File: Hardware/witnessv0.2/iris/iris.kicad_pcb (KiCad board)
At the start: 4 copper layers, 30 x 50 mm, 112 parts, among them J1 Conn_01x02, J2 Conn_01x02, J3 USB_B_Micro, J4 Conn_01x02, J5 Conn_01x04, J6 Conn_01x04, J7 Conn_01x04, J8 Conn_01x04, J9 Conn_01x04, Q1 SQA403EJ, Q2 SQA403EJ, U1 ESP32-S3FN8, U10 RA-01SH-P, U2 TPS63070, U3 INA2180A3IDSG, U4 LSM6DSV320XTR, U5 ICM-45686, U6 TPS63070, U7 MS5607-02BA, U8 W25N01KVZEIR, U9 USBLC6-2SC6, Y1 F322540MUBCE2O

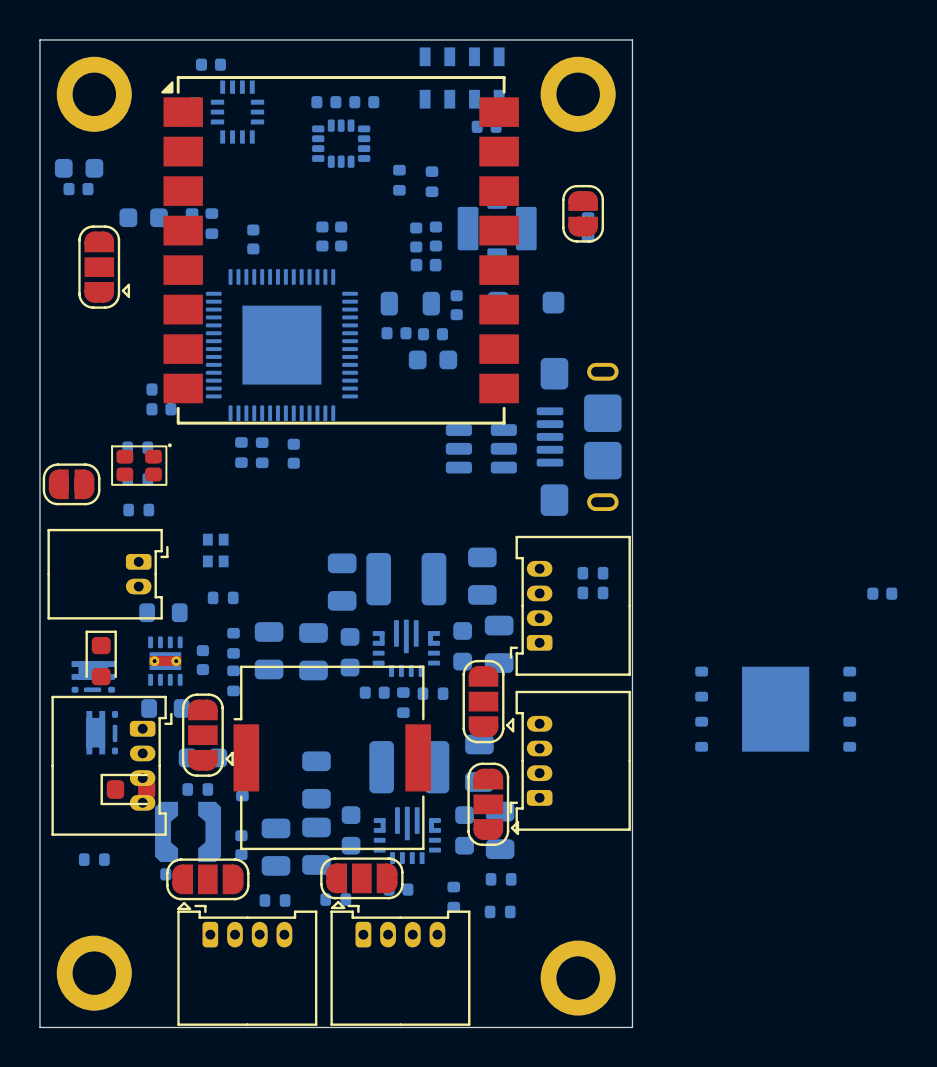
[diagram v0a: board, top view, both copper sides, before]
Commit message: iris rework
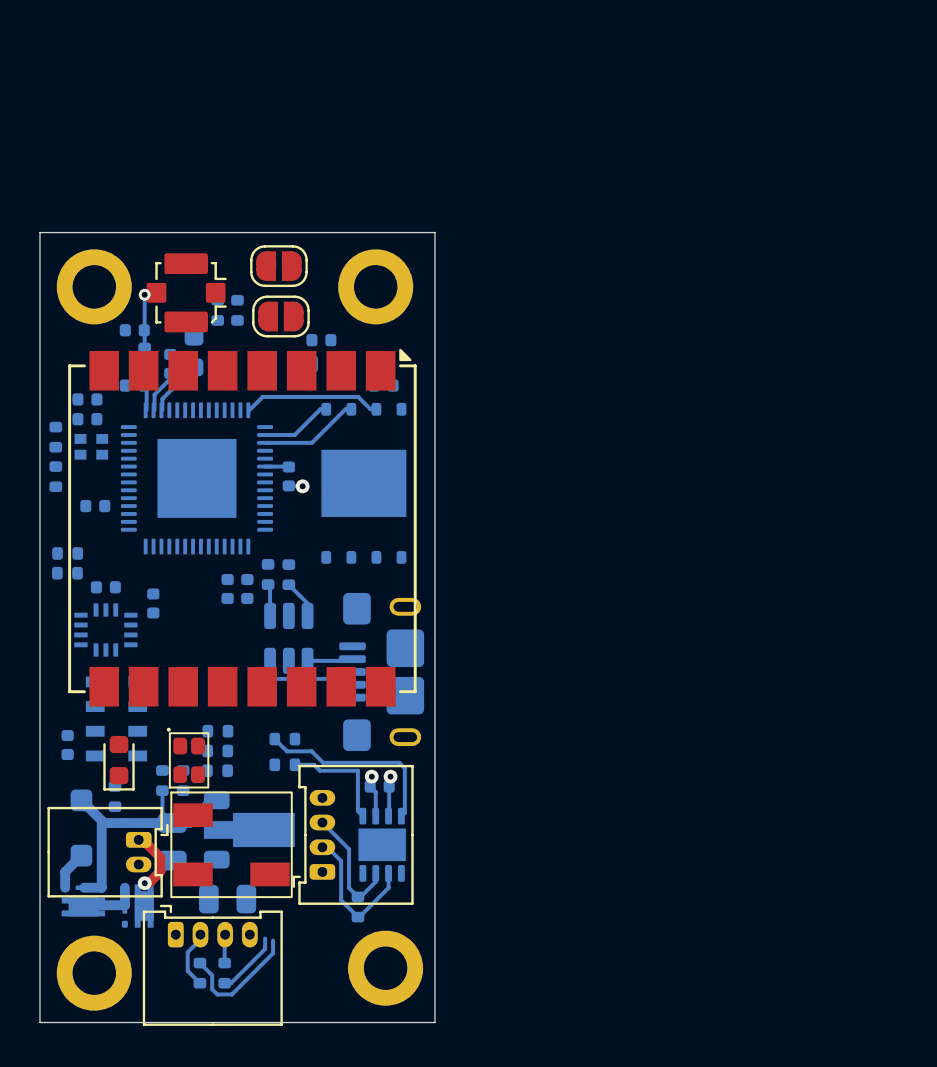
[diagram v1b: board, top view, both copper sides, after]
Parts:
- removed C12, C13, C14, C23, C24, C25: 22u, Capacitor_SMD:C_0805_2012Metric
- removed C15, C16, C21, C29, C34, C39, C40, C7: 100n, Capacitor_SMD:C_0402_1005Metric
- removed C17: 470n, Capacitor_SMD:C_0603_1608Metric
- removed C18, C19: 10u, Capacitor_SMD:C_0805_2012Metric
- removed C20, C22, C43, C8, C9: 10u, Capacitor_SMD:C_0603_1608Metric
- removed D3: LED, LED_SMD:LED_0603_1608Metric
- removed J7, J8, J9: Conn_01x04, Witness:Molex_MicroLock-2200980471-01x04-Horizontal
- removed JP1, JP2, JP3, JP4, JP5, JP6: SolderJumper_3_Open, Jumper:SolderJumper-3_P1.3mm_Open_RoundedPad1.0x1.5mm
- removed L1, L3: 1u, Inductor_SMD:L_1210_3225Metric
- removed L2: 2.2u, Inductor_SMD:L_Coilcraft_LPS3010
- removed L4: 10n, Inductor_SMD:L_0805_2012Metric
- removed R1, R9: 100k, Resistor_SMD:R_0402_1005Metric
- removed R10, R12, R6: 10k, Resistor_SMD:R_0402_1005Metric
- removed R11: 35k, Resistor_SMD:R_0402_1005Metric
- removed R2: 470k, Resistor_SMD:R_0402_1005Metric
- removed R3: 150k, Resistor_SMD:R_0402_1005Metric
- removed R5: 4.7, Resistor_SMD:R_0402_1005Metric
- removed R7: 680k, Resistor_SMD:R_0402_1005Metric
- removed R8: 130k, Resistor_SMD:R_0402_1005Metric
- removed U3: INA2180A3IDSG, Package_SON:Texas_DSG0008A_WSON-8-1EP_2x2mm_P0.5mm_EP0.9x1.6mm_ThermalVias
- removed U6: TPS63070, Witness:RNM0015A
- added R32: 1k, Resistor_SMD:R_0402_1005Metric, B.Cu at (110.2, 126.5)
- added R35: 0, Resistor_SMD:R_0402_1005Metric, B.Cu at (111.1, 136.2)
- added R36: 0, Resistor_SMD:R_0402_1005Metric, B.Cu at (112.3, 136.2)
- added R39: 120, Resistor_SMD:R_0402_1005Metric, B.Cu at (119.1, 132.9)
- AE1: moved to F.Cu
- BZ1: footprint Buzzer_Beeper:Buzzer_Murata_PKMCS0909E -> Witness:OWMB-505020S-40-12D
- R33, R34: value 2.5m -> 0; footprint Resistor_SMD:R_0603_1608Metric -> Resistor_SMD:R_0402_1005Metric
- U2: value TPS63070 -> ME6118A33PG; footprint Witness:RNM0015A -> Package_TO_SOT_SMD:SOT-89-3
- U5: value ICM-45686 -> TCAN1044A-Q1; footprint Package_LGA:LGA-14_3x2.5mm_P0.5mm_LayoutBorder3x4y -> Package_SON:VSON-8-1EP_3x3mm_P0.65mm_EP1.65x2.4mm
- moved C38 37.8 mm to (104.4, 124.7), turned to 90 degrees
- moved U7 36.9 mm to (106.9, 123.4), turned to 0 degrees
- moved U5 35.6 mm to (120.3, 129.8), turned to -90 degrees
- moved D4 34.8 mm to (105.1, 128.9), turned to -90 degrees
- moved C36 27.4 mm to (108.7, 117.5), turned to 90 degrees
- moved C35 27.4 mm to (120.4, 106.5)
- moved U4 27.1 mm to (106.3, 118.9), turned to 0 degrees
- moved C37 24.5 mm to (106.3, 116.7), turned to 0 degrees
- moved R25 24.2 mm to (103.8, 111.1)
- moved U8 23.8 mm to (119.4, 111.5), turned to 90 degrees
- moved R28 23.2 mm to (112.0, 102.7), turned to 90 degrees
- moved R29 23.0 mm to (113.0, 102.7), turned to -90 degrees
- moved C28 23.0 mm to (120.2, 126.8), turned to 180 degrees
- moved R24 21.7 mm to (103.8, 109.1), turned to -90 degrees
- moved R27 18.8 mm to (104.4, 116.0), turned to 0 degrees
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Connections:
- net Net-(J3-D+) renamed /IO/USB_UNSAFE_D+
- net Net-(J3-D-) renamed /IO/USB_UNSAFE_D-
- C10 pad 1: /Power/BATT_POSTSW -> +BATT
- C11 pad 1: /Power/BATT_POSTSW -> +3V3
- C28 pad 1: Net-(C28-Pad1) -> +3V3
- D4 pad 1: Net-(D4-K) -> +BATT
- J2 pad 1: +BATT -> /IO/BATT_RAW
- J5 pad 1: Net-(J5-Pin_1) -> +3V3
- J6 pad 1: Net-(J6-Pin_1) -> /IO/GPIO
- J6 pad 2: /IO/GPIO1 -> /IO/CAN_L
- J6 pad 3: /IO/GPIO2 -> /IO/CAN_H
- Q1 pad 1: Net-(D4-K) -> /IO/BATT_RAW
- Q1 pad 4: /Power/ISENSE+ -> Net-(Q1-S)
- Q2 pad 1: +BATT -> Net-(Q1-S)
- Q2 pad 4: Net-(D4-K) -> +BATT
- R21 pad 1: GND -> /MCU/VSENSE
- R21 pad 2: Net-(D3-K) -> +BATT
- R30 pad 1: /MCU/USB_D- -> /IO/USB_D-
- R31 pad 1: /MCU/USB_D+ -> /IO/USB_D+
- R33 pad 1: /Power/ISENSE+ -> /MCU/CANTX
- R33 pad 2: /Power/BATT_POSTSW -> /IO/CANTX
- R34 pad 1: /Power/5VSENSE+ -> /MCU/CANRX
- R34 pad 2: +5V -> /IO/CANRX
- U1 pad 10: unconnected-(U1-GPIO5-Pad10) -> /MCU/RXD_MCU
- U1 pad 11: unconnected-(U1-GPIO6-Pad11) -> /MCU/RAD_RST
- U1 pad 12: unconnected-(U1-GPIO7-Pad12) -> /MCU/LSM_INT1
- U1 pad 13: unconnected-(U1-GPIO8-Pad13) -> /MCU/LSM_INT2
- U1 pad 14: unconnected-(U1-GPIO9-Pad14) -> /MCU/SPI2_IO3
- U1 pad 15: unconnected-(U1-GPIO10-Pad15) -> /MCU/FLASH_CS
- U1 pad 16: unconnected-(U1-GPIO11-Pad16) -> /MCU/SPI2_IO0
- U1 pad 17: unconnected-(U1-GPIO12-Pad17) -> /MCU/SPI2_CLK
- U1 pad 18: unconnected-(U1-GPIO13-Pad18) -> /MCU/SPI2_IO1
- U1 pad 19: unconnected-(U1-GPIO14-Pad19) -> /MCU/SPI2_IO2
- U1 pad 2: Net-(C28-Pad1) -> +3V3
- U1 pad 21: unconnected-(U1-XTAL_32K_P-Pad21) -> /MCU/SPI3_SCLK
- U1 pad 22: unconnected-(U1-XTAL_32K_N-Pad22) -> /MCU/RAD_CS
- U1 pad 23: unconnected-(U1-GPIO17-Pad23) -> /MCU/SPI3_COPI
- U1 pad 24: unconnected-(U1-GPIO18-Pad24) -> /MCU/SPI3_CIPO
- U1 pad 27: unconnected-(U1-GPIO21-Pad27) -> /MCU/MS56_CS
- U1 pad 3: Net-(C28-Pad1) -> +3V3
- U1 pad 36: unconnected-(U1-SPICLK_N-Pad36) -> /MCU/BUZZER
- U1 pad 37: unconnected-(U1-SPICLK_P-Pad37) -> /MCU/LED_B
- U1 pad 38: unconnected-(U1-GPIO33-Pad38) -> /MCU/I2C_SDA
- U1 pad 39: unconnected-(U1-GPIO34-Pad39) -> /MCU/I2C_SCL
- U1 pad 40: unconnected-(U1-GPIO35-Pad40) -> /MCU/LSM_CS
- U1 pad 41: unconnected-(U1-GPIO36-Pad41) -> /MCU/CANTX
- U1 pad 42: unconnected-(U1-GPIO37-Pad42) -> /MCU/CANRX
- U1 pad 43: unconnected-(U1-GPIO38-Pad43) -> /IO/GPIO
- U1 pad 44: unconnected-(U1-MTCK-Pad44) -> /MCU/RAD_BUSY
- U1 pad 45: unconnected-(U1-MTDO-Pad45) -> /MCU/RAD_RF_EN
- U1 pad 47: unconnected-(U1-MTDI-Pad47) -> /MCU/LED_R
- U1 pad 48: unconnected-(U1-MTMS-Pad48) -> /MCU/LED_G
- U1 pad 6: unconnected-(U1-GPIO1-Pad6) -> /MCU/VSENSE
- U1 pad 7: unconnected-(U1-GPIO2-Pad7) -> /MCU/RAD_DIO1
- U1 pad 9: unconnected-(U1-GPIO4-Pad9) -> /MCU/TXD_MCU
- U10 pad 10: /Radio/RAD_BUSY -> /MCU/RAD_BUSY
- U10 pad 11: /Radio/RAD_RF_EN -> /MCU/RAD_RF_EN
- U10 pad 12: /Radio/SPI1_SCLK -> /MCU/SPI3_SCLK
- U10 pad 13: /Radio/SPI1_CIPO -> /MCU/SPI3_CIPO
- U10 pad 14: /Radio/SPI1_COPI -> /MCU/SPI3_COPI
- U10 pad 15: /Radio/RAD_CS -> /MCU/RAD_CS
- U10 pad 4: /Radio/RAD_RST -> /MCU/RAD_RST
- U10 pad 5: Net-(JP6-C) -> +3V3
- U10 pad 6: /Radio/RAD_DIO1 -> /MCU/RAD_DIO1
- U2 pad 1: Net-(U2-PS/SYNC) -> GND
- U2 pad 2: Net-(U2-PG) -> +3V3
- U2 pad 3: Net-(U2-VAUX) -> +BATT
- U4 pad 1: /Sensors/SPI1_CIPO -> /MCU/SPI3_CIPO
- U4 pad 12: /Sensors/LSM_CS -> /MCU/LSM_CS
- U4 pad 13: /Sensors/I2C_SCL -> /MCU/I2C_SCL
- U4 pad 14: /Sensors/I2C_SDA -> /MCU/I2C_SDA
- U4 pad 2: /Sensors/SPI1_SCLK -> /MCU/SPI3_SCLK
- U4 pad 3: /Sensors/SPI1_COPI -> /MCU/SPI3_COPI
- U4 pad 4: /Sensors/LSM_INT1 -> /MCU/LSM_INT1
- U4 pad 9: /Sensors/LSM_INT2 -> /MCU/LSM_INT2
- U5 pad 1: /Sensors/SPI1_CIPO -> /IO/CANRX
- U5 pad 2: /Sensors/I2C_SDA -> GND
- U5 pad 3: /Sensors/I2C_SCL -> +3V3
- U5 pad 4: /Sensors/ICM_INT1 -> /IO/CANTX
- U5 pad 5: +3V3 -> unconnected-(U5-NC-Pad5)
- U5 pad 6: GND -> /IO/CAN_L
- U5 pad 7: unconnected-(U5-RESV-Pad7) -> /IO/CAN_H
- U5 pad 8: +3V3 -> unconnected-(U5-STB-Pad8)
- U5 pad 9: /Sensors/ICM_INT2 -> (no net)
- U7 pad 4: /Sensors/MS56_CS -> /MCU/MS56_CS
- U7 pad 5: /Sensors/MS56_CS -> /MCU/MS56_CS
- U7 pad 6: /Sensors/SPI1_CIPO -> /MCU/SPI3_CIPO
- U7 pad 7: /Sensors/SPI1_COPI -> /MCU/SPI3_COPI
- U7 pad 8: /Sensors/SPI1_SCLK -> /MCU/SPI3_SCLK
- U8 pad 2: /MCU/SPI3_IO2 -> /MCU/SPI2_IO1
- U8 pad 3: /MCU/SPI3_IO3 -> /MCU/SPI2_IO2
- U8 pad 5: /MCU/SPI2_IO1 -> /MCU/SPI2_IO0
- U8 pad 7: /MCU/SPI3_IO3 -> /MCU/SPI2_IO3
- U8 pad 9: (no net) -> GND
- U9 pad 3: /IO/USB_D+ -> /IO/USB_D-
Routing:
- net +BATT: track 0.00 -> 13.9 mm
- net /IO/CANTX: track 0.00 -> 9.69 mm
- net +3V3: track 0.00 -> 8.29 mm, vias 0 -> 1
- net /IO/CAN_L: track 0.00 -> 7.32 mm
- net /MCU/SPI2_IO3: track 0.00 -> 6.97 mm
- net /MCU/TXD_MCU: track 0.00 -> 6.28 mm
- net /IO/CAN_H: track 0.00 -> 6.15 mm
- net /IO/CANRX: track 0.00 -> 5.72 mm
- net /IO/USB_UNSAFE_D+: track 0.00 -> 5.09 mm
- net /MCU/SPI2_CLK: track 0.00 -> 5.02 mm
- net /MCU/SPI2_IO0: track 0.00 -> 3.58 mm
- net /MCU/RXD_MCU: track 0.00 -> 3.30 mm
- net /IO/BATT_RAW: track 0.00 -> 3.22 mm, vias 0 -> 1
- net Net-(Q1-S): track 0.00 -> 3.02 mm
- net /IO/TXD_MCU: track 0.00 -> 2.98 mm
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- added copper zone on In1.Cu, net +3V3
- added copper zone on In2.Cu, net GND
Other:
- board size 30 x 50 mm -> 20 x 40 mm

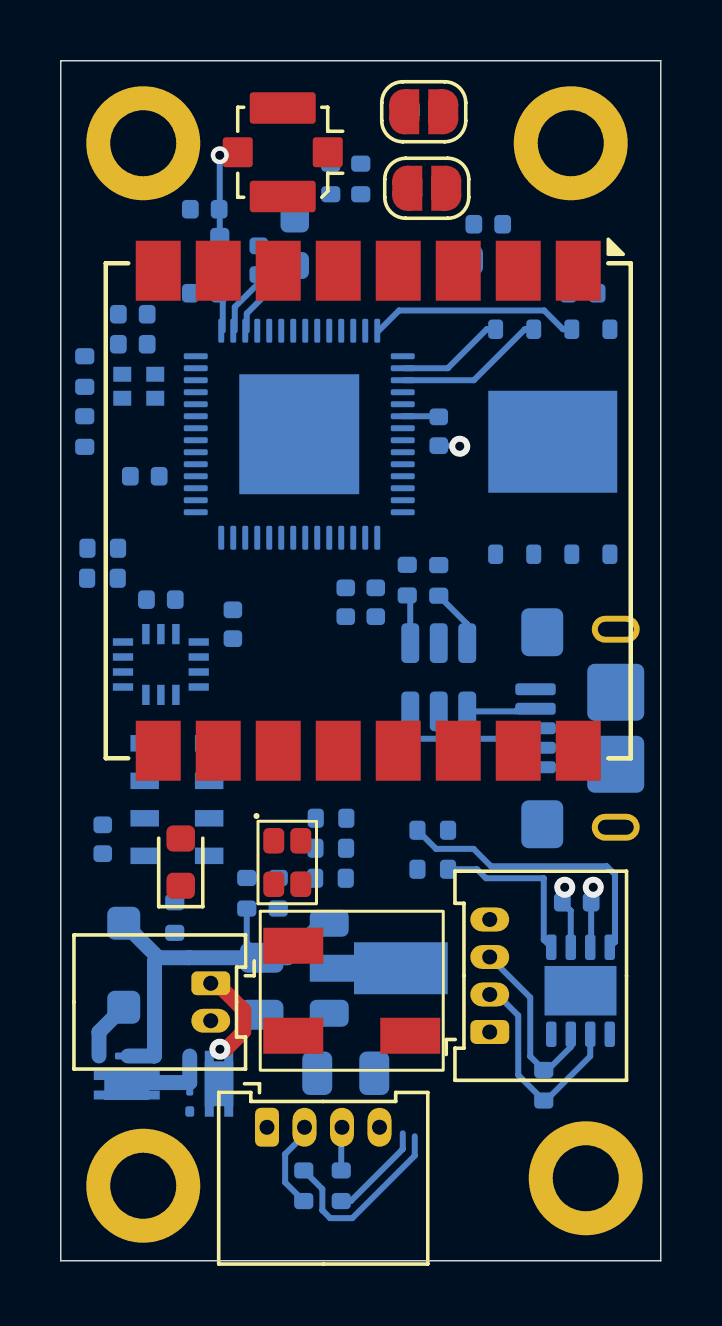
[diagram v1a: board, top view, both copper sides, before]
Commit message: iris inital layout
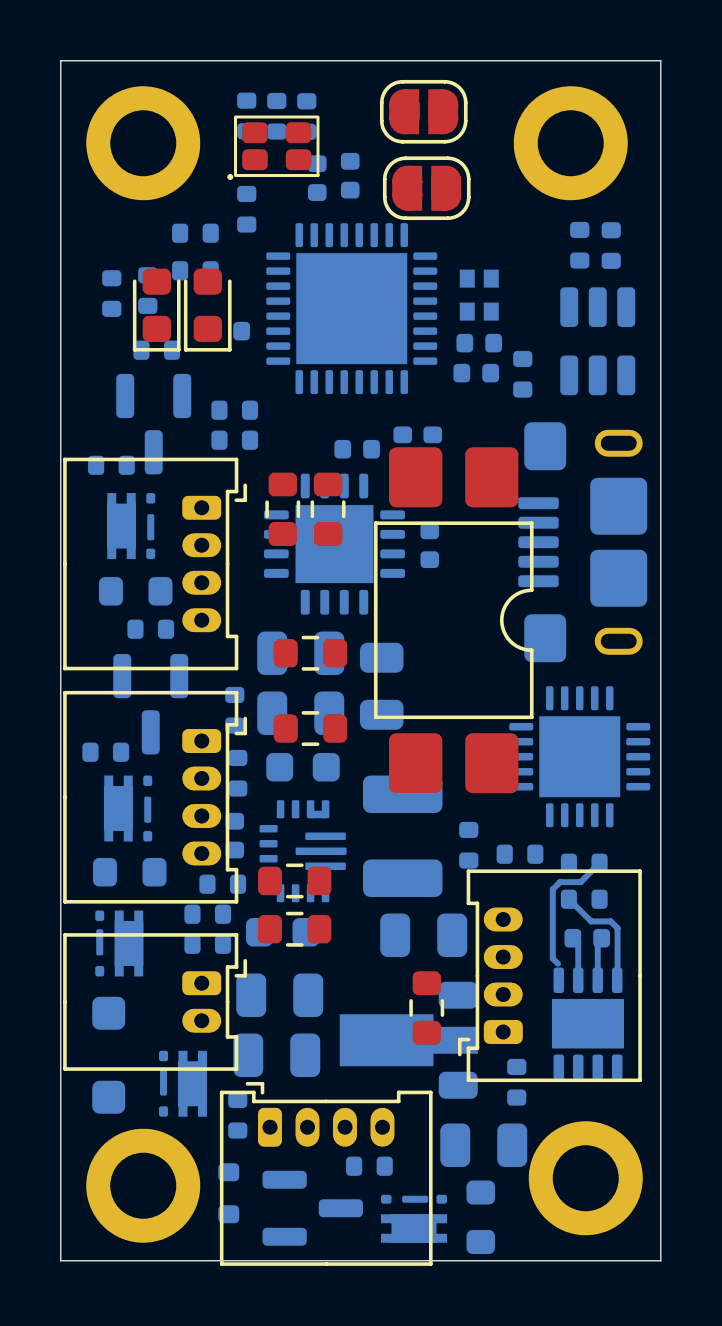
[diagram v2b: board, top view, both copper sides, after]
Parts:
- removed AE1: Antenna_Shield, Connector_Coaxial:U.FL_Molex_MCRF_73412-0110_Vertical
- removed BZ1: Buzzer, Witness:OWMB-505020S-40-12D
- removed C30: 1u, Capacitor_SMD:C_0402_1005Metric
- removed C31, C41: 10u, Capacitor_SMD:C_0603_1608Metric
- removed C32, C33, C35, C36, C37, C38, C42: 100n, Capacitor_SMD:C_0402_1005Metric
- removed L5: L_Small, Inductor_SMD:L_0402_1005Metric
- removed R24, R25, R26, R27, R28, R29: 4.7k, Resistor_SMD:R_0402_1005Metric
- removed U10: RA-01SH-P, RF_Module:Ai-Thinker-Ra-01-LoRa
- removed U8: W25N01KVZEIR, Package_SON:WSON-8-1EP_8x6mm_P1.27mm_EP3.4x4.3mm
- added C18: 10u, Capacitor_SMD:C_0805_2012Metric, B.Cu at (110.3, 129.9)
- added C19: 10u, Capacitor_SMD:C_0805_2012Metric, B.Cu at (110.2, 131.9)
- added C20: 10u, Capacitor_SMD:C_0603_1608Metric, B.Cu at (110.4, 127.8)
- added C21: 100n, Capacitor_SMD:C_0402_1005Metric, B.Cu at (108.8, 124.6)
- added C22: 10u, Capacitor_SMD:C_0603_1608Metric, B.Cu at (111.1, 122.3)
- added C23: 22u, Capacitor_SMD:C_0805_2012Metric, B.Cu at (111.0, 120.5)
- added C24: 22u, Capacitor_SMD:C_0805_2012Metric, B.Cu at (111.0, 118.5)
- added C25: 22u, Capacitor_SMD:C_0805_2012Metric, B.Cu at (113.7, 119.6)
- added C7: 100n, Capacitor_SMD:C_0402_1005Metric, B.Cu at (115.3, 114.9)
- added C8: 100n, Capacitor_SMD:C_0402_1005Metric, B.Cu at (112.9, 111.7)
- added C9: 100n, Capacitor_SMD:C_0402_1005Metric, B.Cu at (108.5, 107.8)
- added D3: LED, LED_SMD:LED_0603_1608Metric, F.Cu at (107.9, 106.9)
- added D5: BZX584C10, Diode_SMD:D_SOD-523, B.Cu at (108.6, 136.5)
- added J7: Conn_01x04, Witness:Molex_MicroLock-2200980471-01x04-Horizontal, F.Cu at (107.7, 113.7)
- added J8: Conn_01x04, Witness:Molex_MicroLock-2200980471-01x04-Horizontal, F.Cu at (107.7, 121.4)
- added L3: 1u, Inductor_SMD:L_1210_3225Metric, B.Cu at (114.4, 124.6)
- added Q11: AO3400A, Package_TO_SOT_SMD:SOT-23, B.Cu at (106.0, 120.2)
- added Q12: SQA403EJ, Package_TO_SOT_SMD:Vishay_PowerPAK_SC70-6L_Single, B.Cu at (105.2, 123.7)
- added Q3: SQA403EJ, Package_TO_SOT_SMD:Vishay_PowerPAK_SC70-6L_Single, B.Cu at (105.3, 114.3)
- added Q4: AO3400A, Package_TO_SOT_SMD:SOT-23, B.Cu at (106.1, 110.9)
- added Q5: AO3400A, Package_TO_SOT_SMD:SOT-23, B.Cu at (111.4, 137.0)
- added Q6: SQA403EJ, Package_TO_SOT_SMD:Vishay_PowerPAK_SC70-6L_Single, B.Cu at (114.8, 137.3)
- added R1: 0, Resistor_SMD:R_0603_1608Metric, F.Cu at (110.4, 113.7)
- added R10: 10k, Resistor_SMD:R_0402_1005Metric, B.Cu at (108.9, 133.9)
- added R11: 0, Resistor_SMD:R_0603_1608Metric, F.Cu at (111.3, 121.0)
- added R13: 0, Resistor_SMD:R_0603_1608Metric, F.Cu at (115.2, 130.3)
- added R2: 0, Resistor_SMD:R_0603_1608Metric, F.Cu at (111.9, 113.7)
- added R3: 0, Resistor_SMD:R_0603_1608Metric, F.Cu at (110.8, 127.7)
- added R38: 1k, Resistor_SMD:R_0402_1005Metric, B.Cu at (105.9, 106.4)
- added R4: 0, Resistor_SMD:R_0603_1608Metric, F.Cu at (110.8, 126.1)
- added R40: 1k, Resistor_SMD:R_0402_1005Metric, B.Cu at (104.7, 112.2)
- added R41: 1k, Resistor_SMD:R_0402_1005Metric, B.Cu at (113.3, 135.6)
- added R42: 1k, Resistor_SMD:R_0402_1005Metric, B.Cu at (108.8, 111.4)
- added R43: 20m, Resistor_SMD:R_0603_1608Metric, B.Cu at (105.5, 116.4)
- added R44: 20m, Resistor_SMD:R_0603_1608Metric, B.Cu at (117.0, 137.3)
- added R45: 1k, Resistor_SMD:R_0402_1005Metric, B.Cu at (108.8, 110.4)
- added R46: 1k, Resistor_SMD:R_0402_1005Metric, B.Cu at (118.4, 109.2)
- added R48: 1k, Resistor_SMD:R_0402_1005Metric, B.Cu at (104.5, 121.8)
- added R49: 20m, Resistor_SMD:R_0603_1608Metric, B.Cu at (105.3, 125.8)
- added R5: 0, Resistor_SMD:R_0603_1608Metric, F.Cu at (111.3, 118.5)
- added R52: 10k, Resistor_SMD:R_0402_1005Metric, B.Cu at (106.2, 108.4)
- added R53: 10k, Resistor_SMD:R_0402_1005Metric, B.Cu at (106.0, 117.7)
- added R54: 10k, Resistor_SMD:R_0402_1005Metric, B.Cu at (118.3, 125.2)
- added R55: 10k, Resistor_SMD:R_0402_1005Metric, B.Cu at (109.2, 103.7)
- added R6: 10k, Resistor_SMD:R_0402_1005Metric, B.Cu at (116.6, 124.9)
- added R7: 680k, Resistor_SMD:R_0402_1005Metric, B.Cu at (108.8, 120.4)
- added R8: 130k, Resistor_SMD:R_0402_1005Metric, B.Cu at (108.9, 122.5)
- added R9: 100k, Resistor_SMD:R_0402_1005Metric, B.Cu at (108.4, 126.2)
- added U3: LTV-817S, Package_DIP:SMDIP-4_W9.53mm, F.Cu at (116.1, 117.4)
- added U6: TPS63070, Witness:RNM0015A, B.Cu at (111.1, 125.1)
- U1: value ESP32-S3FN8 -> PAC1934x-xJQ; footprint Package_DFN_QFN:QFN-56-1EP_7x7mm_P0.4mm_EP4x4mm -> Package_DFN_QFN:UQFN-16-1EP_4x4mm_P0.65mm_EP2.6x2.6mm
- U4: value LSM6DSV320XTR -> MCP23008-xML; footprint Package_LGA:Bosch_LGA-14_3x2.5mm_P0.5mm -> Package_DFN_QFN:QFN-20-1EP_4x4mm_P0.5mm_EP2.7x2.7mm
- U7: value MS5607-02BA -> ESP32-C3FH4; footprint Package_LGA:LGA-8_3x5mm_P1.25mm -> Package_DFN_QFN:QFN-32-1EP_5x5mm_P0.5mm_EP3.7x3.7mm
- moved R35 32.0 mm to (107.5, 104.5), turned to 180 degrees
- moved R36 30.9 mm to (107.5, 105.8), turned to 0 degrees
- moved R19 25.4 mm to (111.2, 100.6), turned to -90 degrees
- moved R18 24.5 mm to (110.2, 100.6), turned to -90 degrees
- moved D1 23.9 mm to (110.2, 101.6), turned to 180 degrees
- moved R17 23.6 mm to (109.2, 100.6), turned to -90 degrees
- moved R20 20.9 mm to (104.7, 106.5), turned to -90 degrees
- moved D2 18.6 mm to (106.2, 106.9)
- moved U7 17.4 mm to (112.7, 107.0), turned to 90 degrees
- moved U4 14.3 mm to (120.3, 122.0), turned to 180 degrees
- moved C6 14.2 mm to (112.7, 102.6), turned to 90 degrees
- moved R30 12.6 mm to (121.3, 104.9)
- moved R31 12.6 mm to (120.3, 104.9)
- moved U9 12.4 mm to (120.9, 108.1)
- moved C3 12.0 mm to (117.0, 108.2), turned to 0 degrees
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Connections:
- net /IO/RXD_MCU renamed /IO/RXD1_MCU
- net /IO/TXD_MCU renamed /IO/TXD1_MCU
- J4 pad 1: /MCU/GPIO0 -> /MCU/LED_G
- J5 pad 1: +3V3 -> /IO/OUT1PWR
- J6 pad 1: /IO/GPIO -> Net-(J6-Pin_1)
- Q1 pad 3: GND -> Net-(D5-A)
- R23 pad 1: /MCU/GPIO0 -> /MCU/LED_G
- R30 pad 2: Net-(U1-GPIO19/USB_D-) -> Net-(U7-GPIO18)
- R31 pad 2: Net-(U1-GPIO20/USB_D+) -> Net-(U7-GPIO19)
- R35 pad 1: /MCU/TXD_MCU -> /MCU/TXD1_MCU
- R36 pad 1: /MCU/RXD_MCU -> /MCU/RXD1_MCU
- U1 pad 1: Net-(U1-LNA_IN) -> GND
- U1 pad 10: /MCU/RXD_MCU -> unconnected-(U1-SENSE4+-Pad10)
- U1 pad 11: /MCU/RAD_RST -> /Load Switches/VIN1
- U1 pad 12: /MCU/LSM_INT1 -> /Load Switches/CS1
- U1 pad 13: /MCU/LSM_INT2 -> /Load Switches/VIN1
- U1 pad 14: /MCU/SPI2_IO3 -> /Load Switches/CS2
- U1 pad 15: /MCU/FLASH_CS -> +3V3
- U1 pad 16: /MCU/SPI2_IO0 -> GND
- U1 pad 17: /MCU/SPI2_CLK -> GND
- U1 pad 3: +3V3 -> GND
- U1 pad 4: /MCU/RST -> /Load Switches/SCL
- U1 pad 5: /MCU/GPIO0 -> /Load Switches/SDA
- U1 pad 6: /MCU/VSENSE -> GND
- U1 pad 7: /MCU/RAD_DIO1 -> /Load Switches/CS3
- U1 pad 8: /MCU/GPIO3 -> /Load Switches/VIN1
- U1 pad 9: /MCU/TXD_MCU -> unconnected-(U1-SENSE4--Pad9)
- U4 pad 1: /MCU/SPI3_CIPO -> GND
- U4 pad 10: unconnected-(U4-OCS_aux-Pad10) -> /Load Switches/EN2
- U4 pad 11: unconnected-(U4-SDO_aux-Pad11) -> /Load Switches/EN3
- U4 pad 12: /MCU/LSM_CS -> /MCU/5V_EN
- U4 pad 13: /MCU/I2C_SCL -> unconnected-(U4-GP4-Pad13)
- U4 pad 14: /MCU/I2C_SDA -> unconnected-(U4-GP5-Pad14)
- U4 pad 2: /MCU/SPI3_SCLK -> GND
- U4 pad 3: /MCU/SPI3_COPI -> GND
- U4 pad 4: /MCU/LSM_INT1 -> /MCU/LS_EN
- U4 pad 5: +3V3 -> unconnected-(U4-NC-Pad5)
- U4 pad 6: GND -> unconnected-(U4-NC-Pad6)
- U4 pad 7: GND -> unconnected-(U4-INT-Pad7)
- U4 pad 8: +3V3 -> unconnected-(U4-NC-Pad8)
- U4 pad 9: /MCU/LSM_INT2 -> /Load Switches/EN1
- U7 pad 1: +3V3 -> unconnected-(U7-LNA_IN-Pad1)
- U7 pad 2: GND -> +3V3
- U7 pad 3: GND -> +3V3
- U7 pad 4: /MCU/MS56_CS -> /MCU/VSENSE
- U7 pad 5: /MCU/MS56_CS -> /MCU/CANTX
- U7 pad 6: /MCU/SPI3_CIPO -> /IO/BUTTON
- U7 pad 7: /MCU/SPI3_COPI -> /MCU/RST
- U7 pad 8: /MCU/SPI3_SCLK -> /MCU/CANRX
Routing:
- net +BATT: track 13.9 -> 0.00 mm
- net /IO/CAN_L: track 7.32 -> 0.00 mm
- net /MCU/SPI2_IO3: track 6.97 -> 0.00 mm
- net +3V3: track 8.29 -> 1.45 mm, vias 1 -> 0
- net /MCU/TXD_MCU: track 6.28 -> 0.00 mm
- net /IO/CAN_H: track 6.15 -> 0.00 mm
- net /IO/CANTX: track 9.69 -> 3.76 mm
- net /IO/USB_UNSAFE_D+: track 5.09 -> 0.00 mm
- net /MCU/SPI2_CLK: track 5.02 -> 0.00 mm
- net /MCU/SPI2_IO0: track 3.58 -> 0.00 mm
- net /MCU/RXD_MCU: track 3.30 -> 0.00 mm
- net /IO/BATT_RAW: track 3.22 -> 0.00 mm, vias 1 -> 0
- net Net-(D5-K): track 3.02 -> 0.00 mm
- net /IO/TXD1_MCU: track 2.98 -> 0.00 mm
- net Net-(AE1-A): track 2.71 -> 0.00 mm, vias 1 -> 0
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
